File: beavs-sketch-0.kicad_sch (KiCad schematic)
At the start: 17 parts, among them J1 USB_C_Receptacle_USB2.0_16P, J3 Conn_01x02, J4 Conn_Coaxial, J5 Conn_01x02, Q2 SiS427EDN, U4 RFM95W-915S2, U7 AMS1117-3.3, U8 AMS1117-5.0

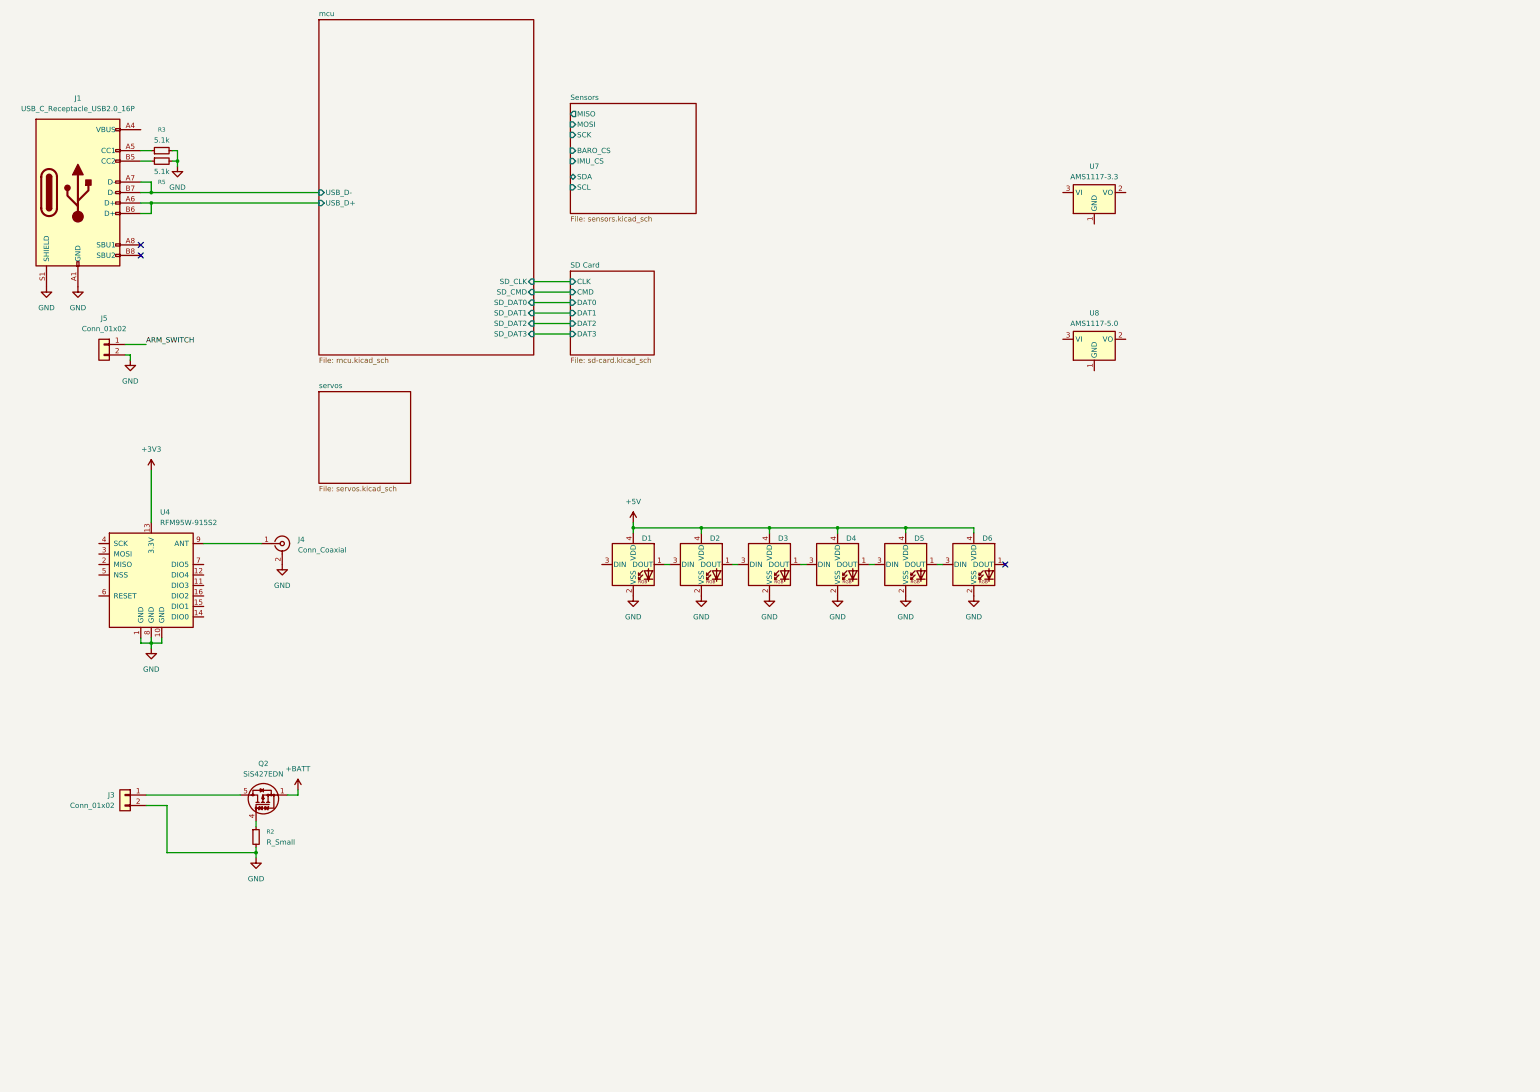
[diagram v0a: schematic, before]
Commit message: add 3d models and do other stuff
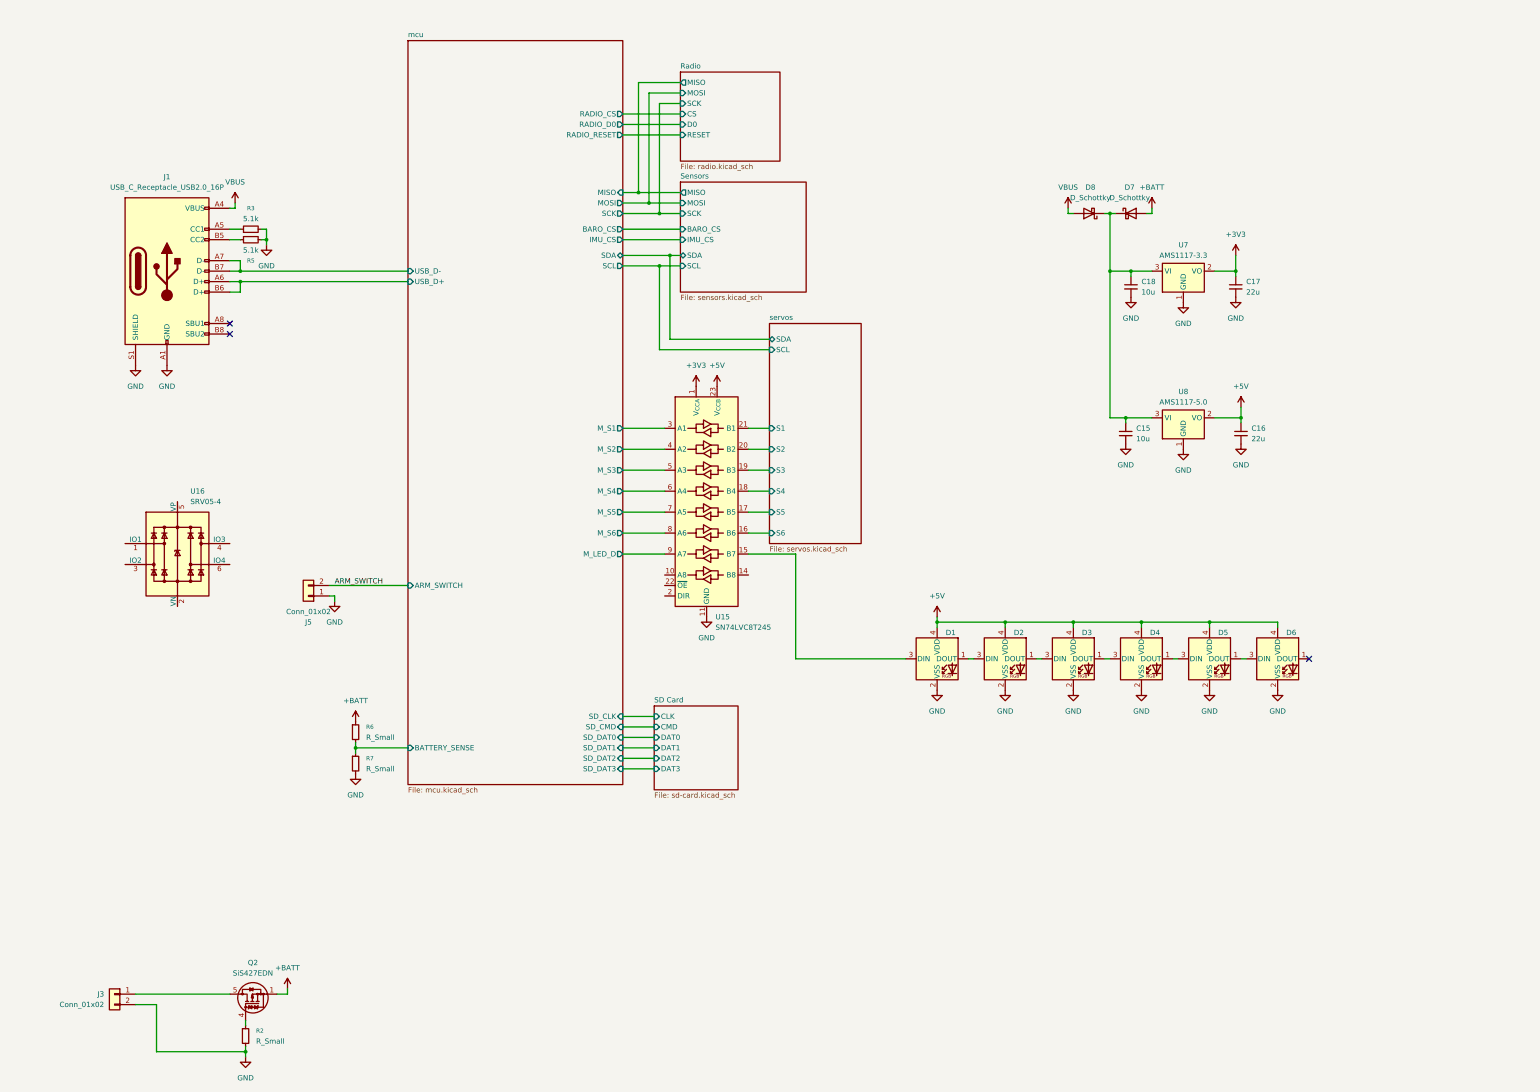
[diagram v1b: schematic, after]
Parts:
- removed J4: Conn_Coaxial, Connector_Coaxial:U.FL_Molex_MCRF_73412-0110_Vertical, symbol Connector:Conn_Coaxial
- removed U4: RFM95W-915S2, RF_Module:HOPERF_RFM9XW_SMD, symbol RF_Module:RFM95W-915S2
- added C15, C18: 10u, Capacitor_SMD:C_0603_1608Metric, symbol Device:C_Small
- added C16, C17: 22u, Capacitor_SMD:C_0603_1608Metric, symbol Device:C_Small
- added D7, D8: D_Schottky, Diode_SMD:D_SOD-123, symbol Device:D_Schottky
- added R6, R7: R_Small, Resistor_SMD:R_0402_1005Metric, symbol Device:R_Small
- added U15: SN74LVC8T245, Package_SO:TSSOP-24_4.4x7.8mm_P0.65mm, symbol Logic_LevelTranslator:SN74LVC8T245
- added U16: SRV05-4, Package_TO_SOT_SMD:SOT-23-6, symbol Power_Protection:SRV05-4
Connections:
- net +3V3: now also U7.2 (VO), C17.1, U15.1 (V_{CCA})
- net +5V: now also U8.2 (VO), C16.1, U15.23 (V_{CCB}), U15.24 (V_{CCB})
- net +BATT: now also D7.2 (A), R6.1
- net ARM_SWITCH: now also J5.2 (Pin_2); no longer J5.1 (Pin_1)
- net GND: now also J5.1 (Pin_1), U7.1 (GND), U8.1 (GND), C15.2, C16.2, C17.2, C18.2, R7.2, U15.11 (GND), U15.12 (GND), U15.13 (GND); no longer J5.2 (Pin_2)
- net at U8.3 (VI): now also U7.3 (VI), C15.1, C18.1, D7.1 (K), D8.1 (K)
- net VBUS: now reaches J1.A4 (VBUS), J1.A9 (VBUS), J1.B4 (VBUS), J1.B9 (VBUS)
- net VBUS: now also D8.2 (A)
- net at D1.3 (DIN): now also U15.15 (B7)
- new net mcu/BATTERY_SENSE: R6.2, R7.1
- new net mcu/M_LED_D: U15.9 (A7)
- new net mcu/M_S1: U15.3 (A1)
- new net mcu/M_S2: U15.4 (A2)
- new net mcu/M_S3: U15.5 (A3)
- new net mcu/M_S4: U15.6 (A4)
- new net mcu/M_S5: U15.7 (A5)
- new net mcu/M_S6: U15.8 (A6)
- new net servos/S1: U15.21 (B1)
- new net servos/S2: U15.20 (B2)
- new net servos/S3: U15.19 (B3)
- new net servos/S4: U15.18 (B4)
- new net servos/S5: U15.17 (B5)
- new net servos/S6: U15.16 (B6)
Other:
- added sheet Radio (radio.kicad_sch)
- sheet mcu ports: added ARM_SWITCH, BARO_CS, BATTERY_SENSE, IMU_CS, MISO, MOSI, M_LED_D, M_S1, M_S2, M_S3, M_S4, M_S5, M_S6, RADIO_CS, RADIO_D0, RADIO_RESET, SCK, SCL, SDA; removed none
- sheet servos ports: added S1, S2, S3, S4, S5, S6, SCL, SDA; removed none
- moved on the sheet: D1, D2, D3, D4, D5, D6, J1, J3, J5, Q2, R2, R3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

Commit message: add some TVS diodes
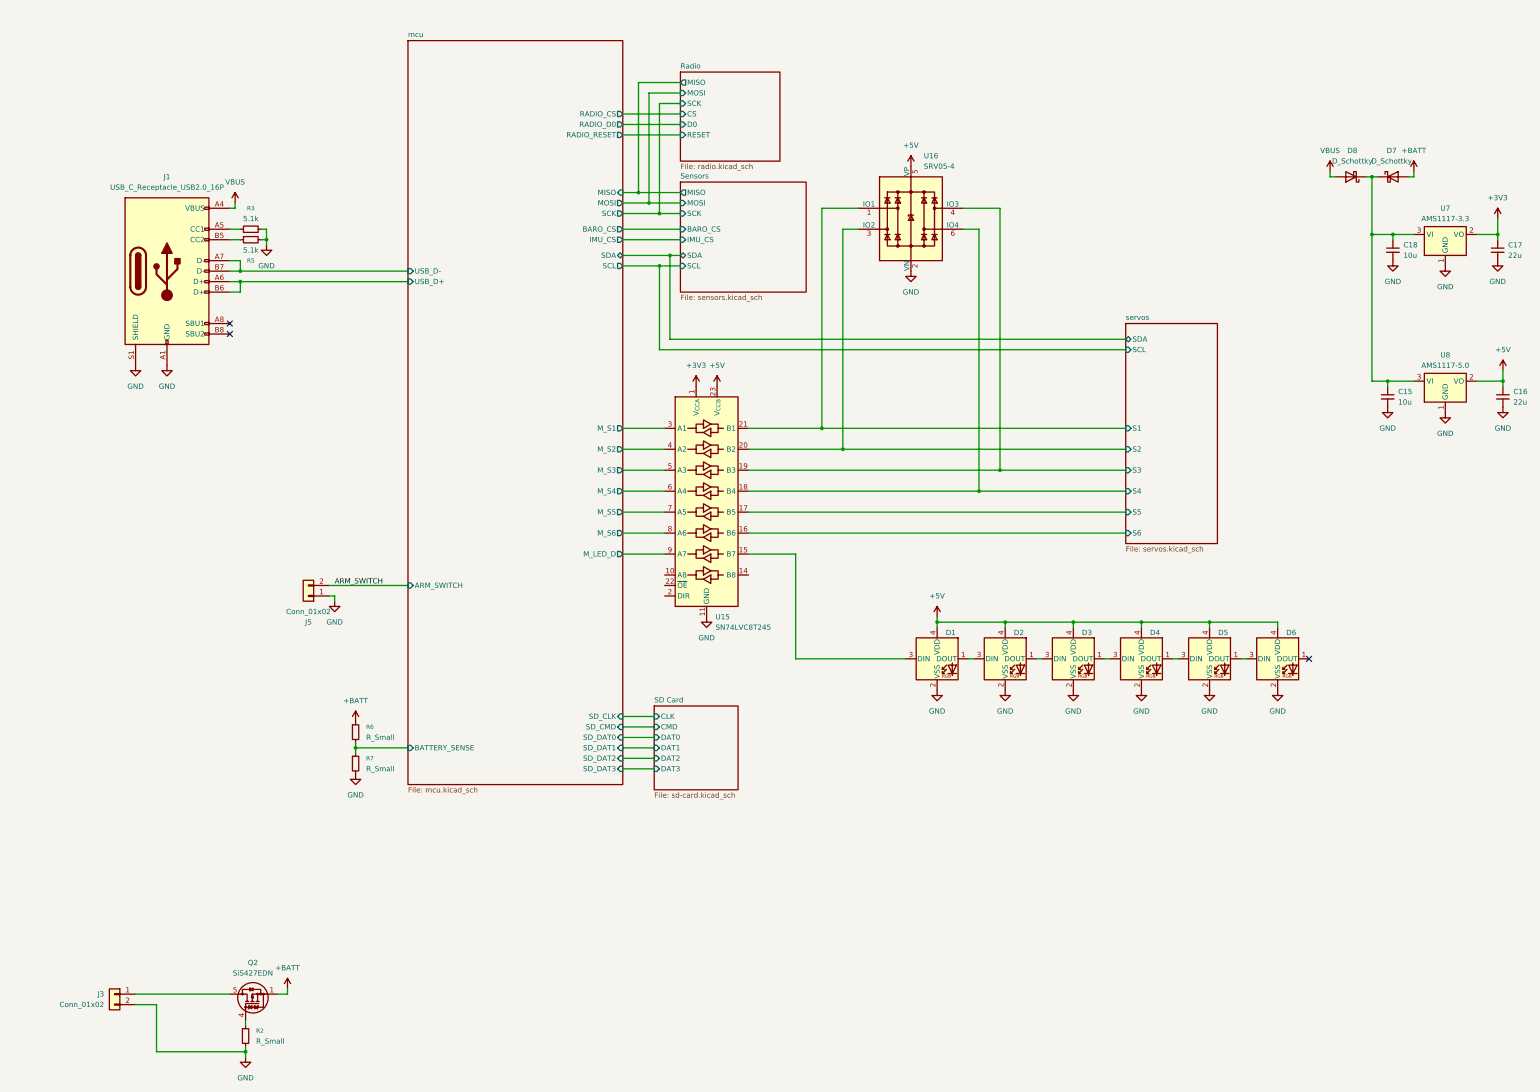
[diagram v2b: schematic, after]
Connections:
- net +5V: now also U16.5 (VP)
- net GND: now also U16.2 (VN)
- net servos/S1: now also U16.1 (IO1)
- net servos/S2: now also U16.3 (IO2)
- net servos/S3: now also U16.4 (IO3)
- net servos/S4: now also U16.6 (IO4)
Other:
- moved on the sheet: C15, C16, C17, C18, D7, D8, U16, U7, U8
